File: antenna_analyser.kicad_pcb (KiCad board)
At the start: 2 copper layers, 99.7 x 50.8 mm, 31 parts, among them IC1 MCP6002, IC2 ARDUINO_PRO_MINI_3.3V, P1 AD9850_CONN, P2 CONN_LCD, U1 AMS1117

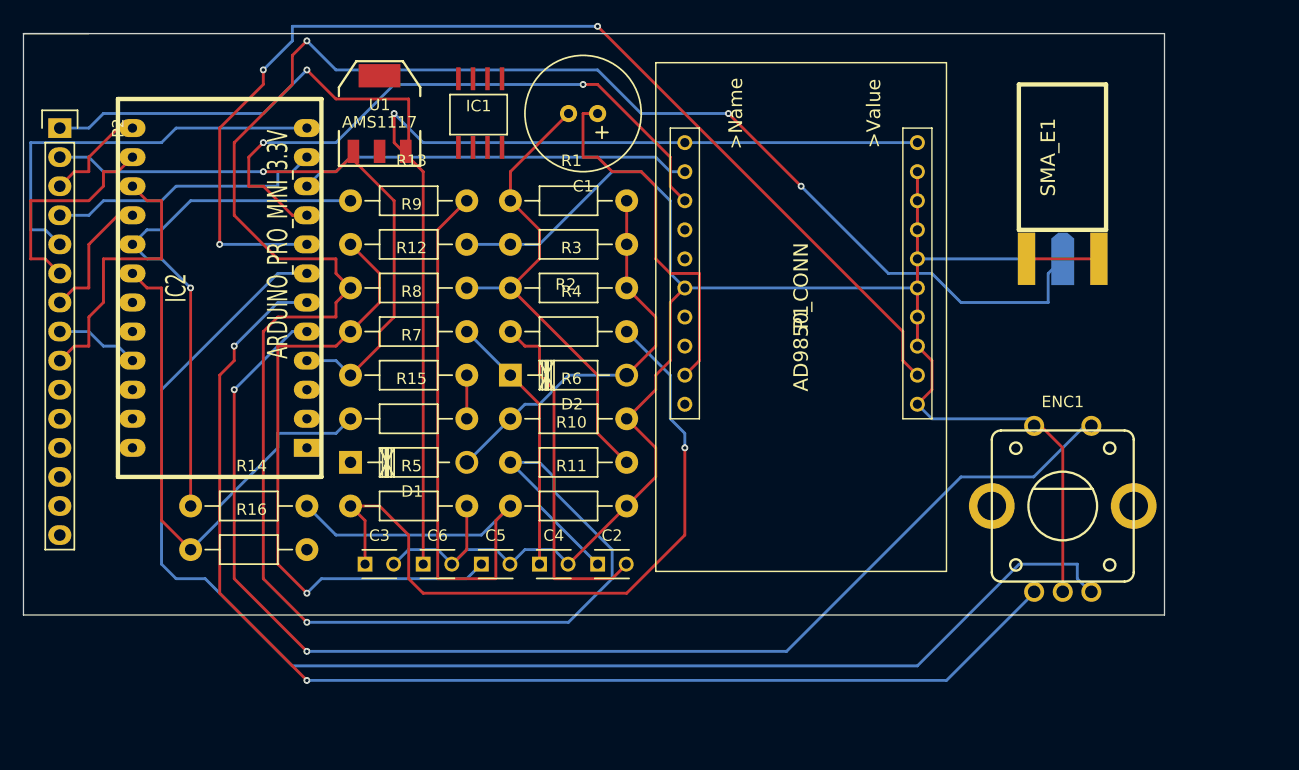
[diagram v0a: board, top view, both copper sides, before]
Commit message: WIP
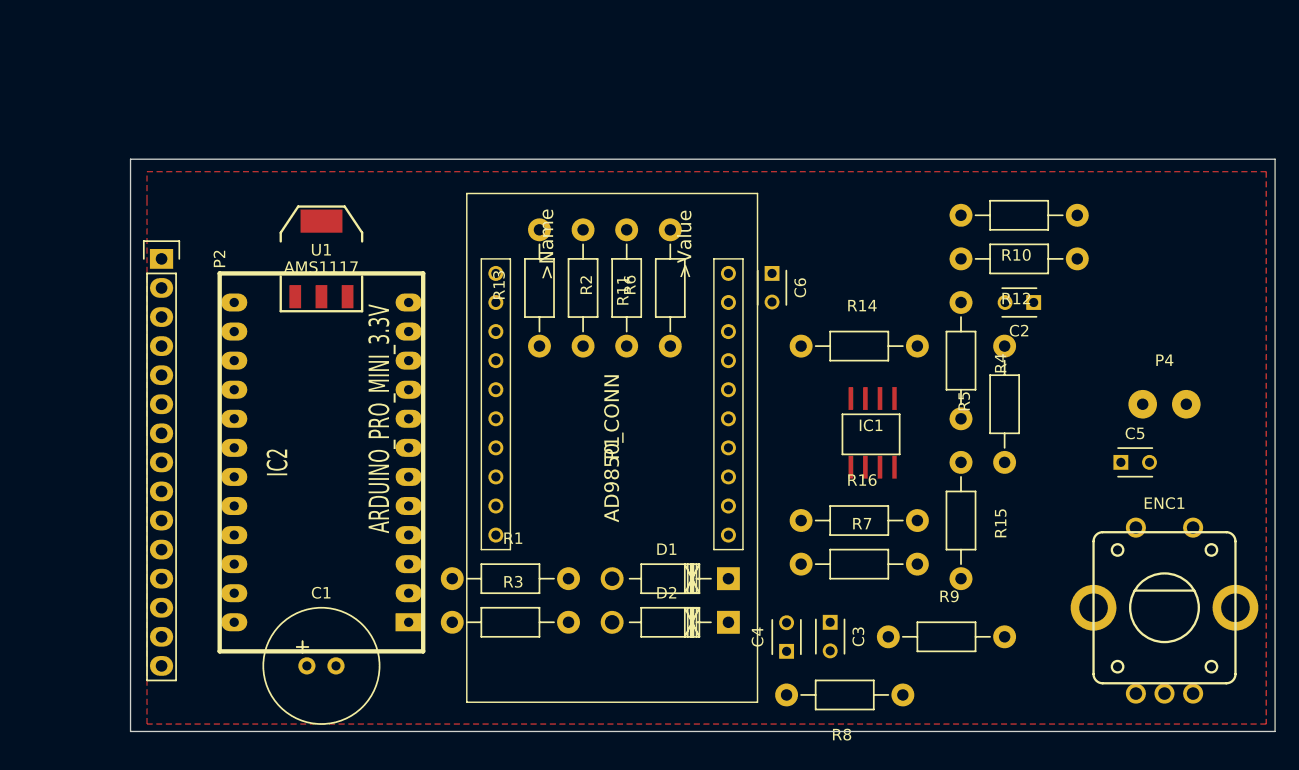
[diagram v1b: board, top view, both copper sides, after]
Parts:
- removed SMA_E1: SMA_EDGE, SMA_EDGE:SMA_EDGE
- added P4: BNC, Wire_Pads:SolderWirePad_2x_1mmDrill, F.Cu at (180.3, 105.4)
- moved R9 58.2 mm to (161.3, 125.7)
- moved C5 56.6 mm to (176.5, 110.5)
- moved R14 55.1 mm to (153.7, 100.3)
- moved C1 54.5 mm to (105.4, 128.3), turned to 0 degrees
- moved R12 53.4 mm to (167.6, 92.7), turned to 180 degrees
- moved R16 53.4 mm to (153.7, 115.6)
- moved R5 52.8 mm to (166.4, 105.4), turned to 90 degrees
- moved R8 49.6 mm to (152.4, 130.8), turned to 180 degrees
- moved R15 49.1 mm to (162.6, 115.6), turned to 270 degrees
- moved R10 44.9 mm to (167.6, 88.9), turned to 180 degrees
- moved C2 44.4 mm to (168.9, 96.5), turned to 180 degrees
- moved IC1 44.2 mm to (152.4, 105.4)
- moved R7 42.7 mm to (153.7, 119.4)
- moved C3 41.0 mm to (151.1, 124.5), turned to 270 degrees
- moved C6 39.7 mm to (146.1, 94.0), turned to 270 degrees
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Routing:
- net GND: track 225.4 -> 0.00 mm, vias 1 -> 0
- net Net-(C2-Pad1): track 202.8 -> 0.00 mm, vias 4 -> 0
- net +5V: track 127.6 -> 0.00 mm, vias 2 -> 0
- net Net-(ENC1-PadB): track 122.7 -> 0.00 mm
- net Net-(ENC1-PadSW2): track 111.6 -> 0.00 mm, vias 2 -> 0
- net Net-(ENC1-PadA): track 107.6 -> 0.00 mm, vias 2 -> 0
- net Net-(IC2-Pad8): track 98.0 -> 0.00 mm, vias 3 -> 0
- net Net-(IC1-Pad6): track 65.9 -> 0.00 mm
- net Net-(C3-Pad1): track 62.2 -> 0.00 mm, vias 1 -> 0
- net Net-(C5-Pad1): track 55.5 -> 0.00 mm, vias 1 -> 0
- net Net-(IC2-Pad9): track 55.1 -> 0.00 mm, vias 2 -> 0
- net Net-(IC1-Pad1): track 47.2 -> 0.00 mm
- net Net-(IC1-Pad7): track 46.3 -> 0.00 mm, vias 1 -> 0
- net Net-(C1-Pad2): track 42.7 -> 0.00 mm
- net Net-(IC2-Pad12): track 35.3 -> 0.00 mm
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- added copper zone on F.Cu, net GND
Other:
- board size 99.7 x 50.8 mm -> 100 x 50 mm
